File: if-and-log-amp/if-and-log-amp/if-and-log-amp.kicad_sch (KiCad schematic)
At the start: 84 parts, among them J301 Coax, J302 SMA Panel Mount, J303 SMA Panel Mount, J304 SMA Panel Mount, J305 Conn_01x03, J306 Conn_01x02, J307 Conn_Coaxial, Q301 2N3904, T301 FT37-43 8:2 t, U301 AD603AQ, U302 L78L05_TO92, U303 LM317L_TO92, U304 AD8307AN, U305 CA3140

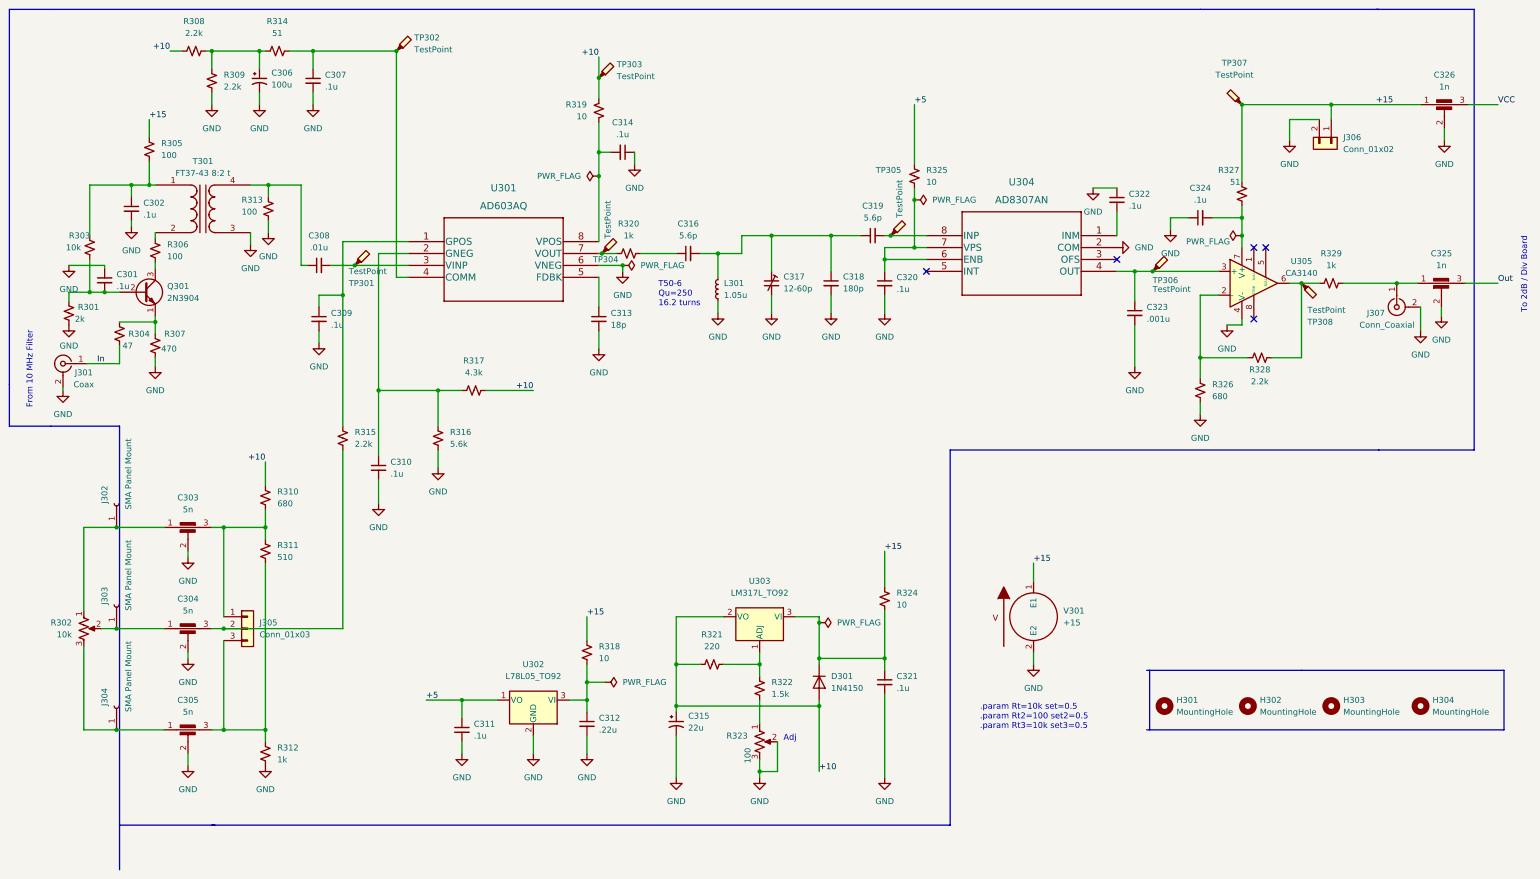
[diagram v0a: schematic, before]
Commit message: v7 conversion
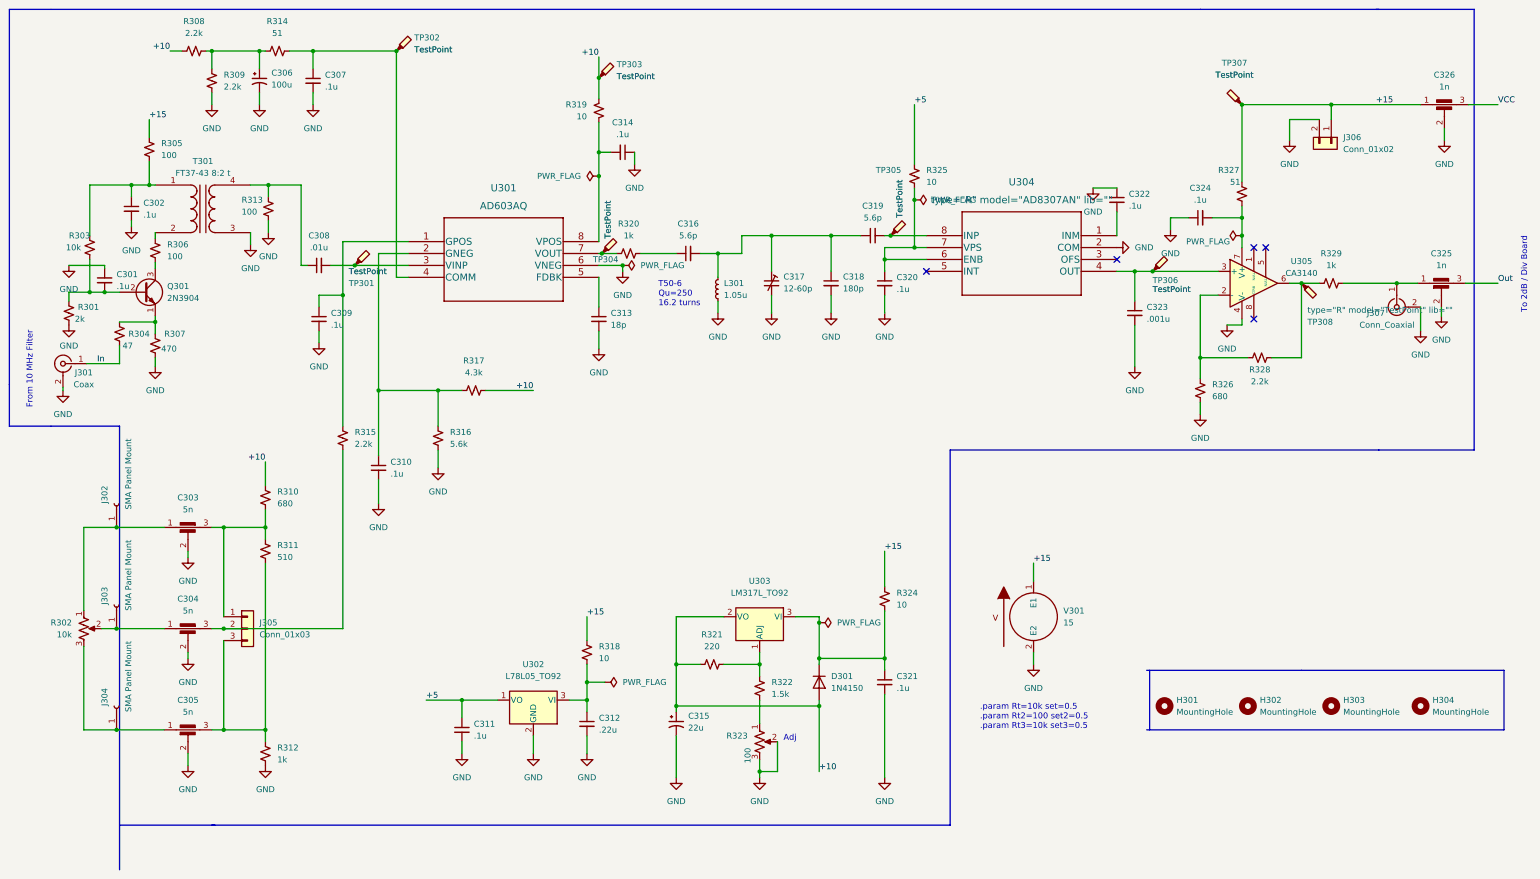
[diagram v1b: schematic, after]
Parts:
- D301: Spice_Lib_File if-log-amp-spice\fairch.lib -> (none); Spice_Model 1N4152 -> (none); Spice_Netlist_Enabled Y -> (none); Spice_Node_Sequence 2 1 -> (none); Spice_Primitive D -> (none)
- J301, J307: Spice_Model Conn_Coaxial -> (none); Spice_Netlist_Enabled N -> (none); Spice_Primitive J -> (none)
- J302, J303, J304: Spice_Model SMA Panel Mount -> (none); Spice_Netlist_Enabled N -> (none); Spice_Primitive J -> (none)
- R302: Spice_Lib_File if-log-amp-spice\Pot.lib -> (none); Spice_Model pot_alps_a -> (none); Spice_Netlist_Enabled Y -> (none); Spice_Primitive X -> (none)
- R323: Spice_Lib_File if-log-amp-spice\Pot2.lib -> (none); Spice_Model pot_lin2 -> (none); Spice_Netlist_Enabled Y -> (none); Spice_Primitive X -> (none)
- TP301, TP302, TP303, TP304, TP305, TP306, TP307: value TestPoint -> ${SIM.PARAMS}; Spice_Netlist_Enabled N -> (none)
- TP308: value TestPoint -> ${SIM.PARAMS}; Spice_Netlist_Enabled N -> (none); Spice_Primitive R -> (none)
- U301: Spice_Lib_File if-log-amp-spice\ad603a.cir -> (none); Spice_Model AD603A -> (none); Spice_Netlist_Enabled Y -> (none); Spice_Primitive X -> (none)
- U302: Spice_Lib_File if-log-amp-spice\78L05_TEST.sub -> (none); Spice_Model X78L05 -> (none); Spice_Netlist_Enabled Y -> (none); Spice_Node_Sequence 3 2 1 -> (none); Spice_Primitive X -> (none)
- U303: Spice_Lib_File if-log-amp-spice\lm317.lib -> (none); Spice_Model LM317TI -> (none); Spice_Netlist_Enabled Y -> (none); Spice_Node_Sequence 3 1 2 -> (none); Spice_Primitive X -> (none)
- U304: value AD8307AN -> ${SIM.PARAMS}; Spice_Netlist_Enabled N -> (none); Spice_Primitive R -> (none)
- U305: Spice_Lib_File if-log-amp-spice\ca3140.sub -> (none); Spice_Model ca3140 -> (none); Spice_Netlist_Enabled Y -> (none); Spice_Primitive X -> (none)
- V301: value +15 -> 15; Spice_Model dc 15 -> (none); Spice_Netlist_Enabled Y -> (none); Spice_Primitive V -> (none)
